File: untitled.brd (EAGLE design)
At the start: 100 x 100 mm, 16 parts, among them X2 pzem-004t

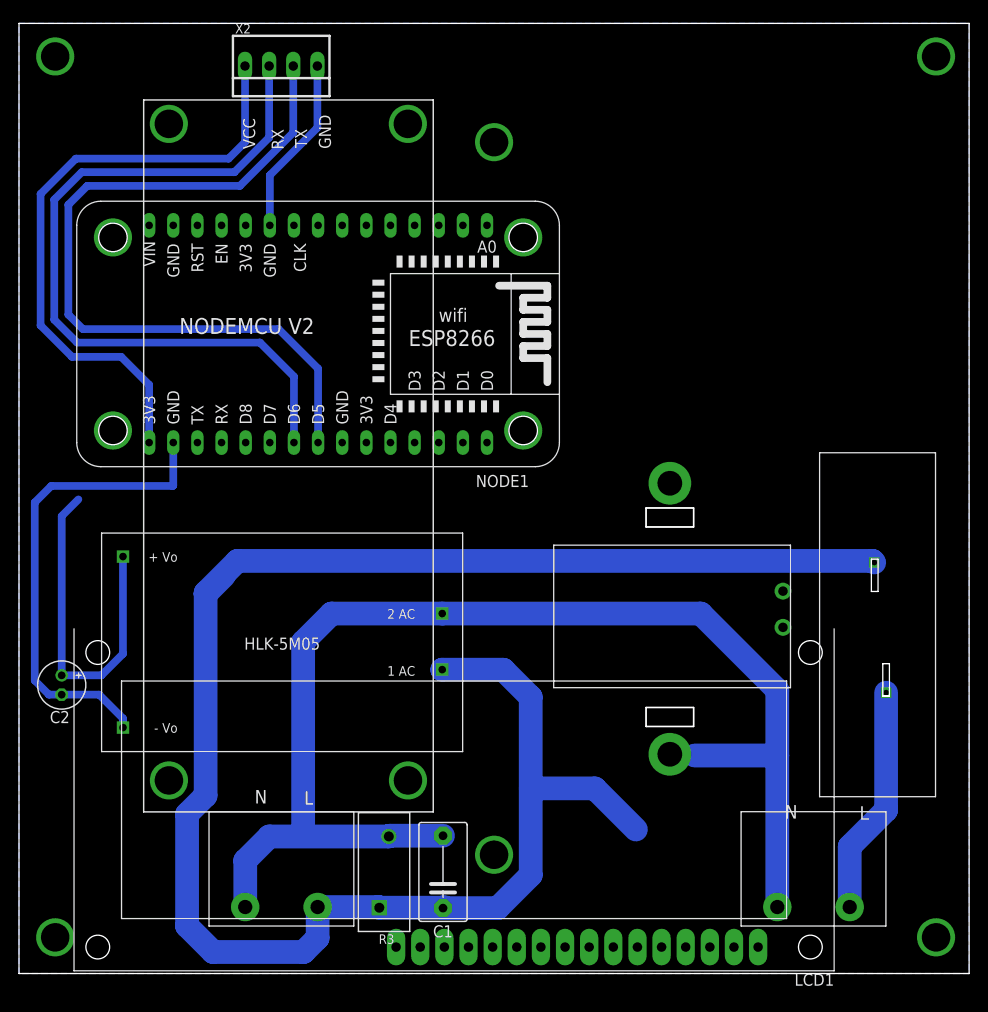
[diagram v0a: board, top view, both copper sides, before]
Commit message: 0021
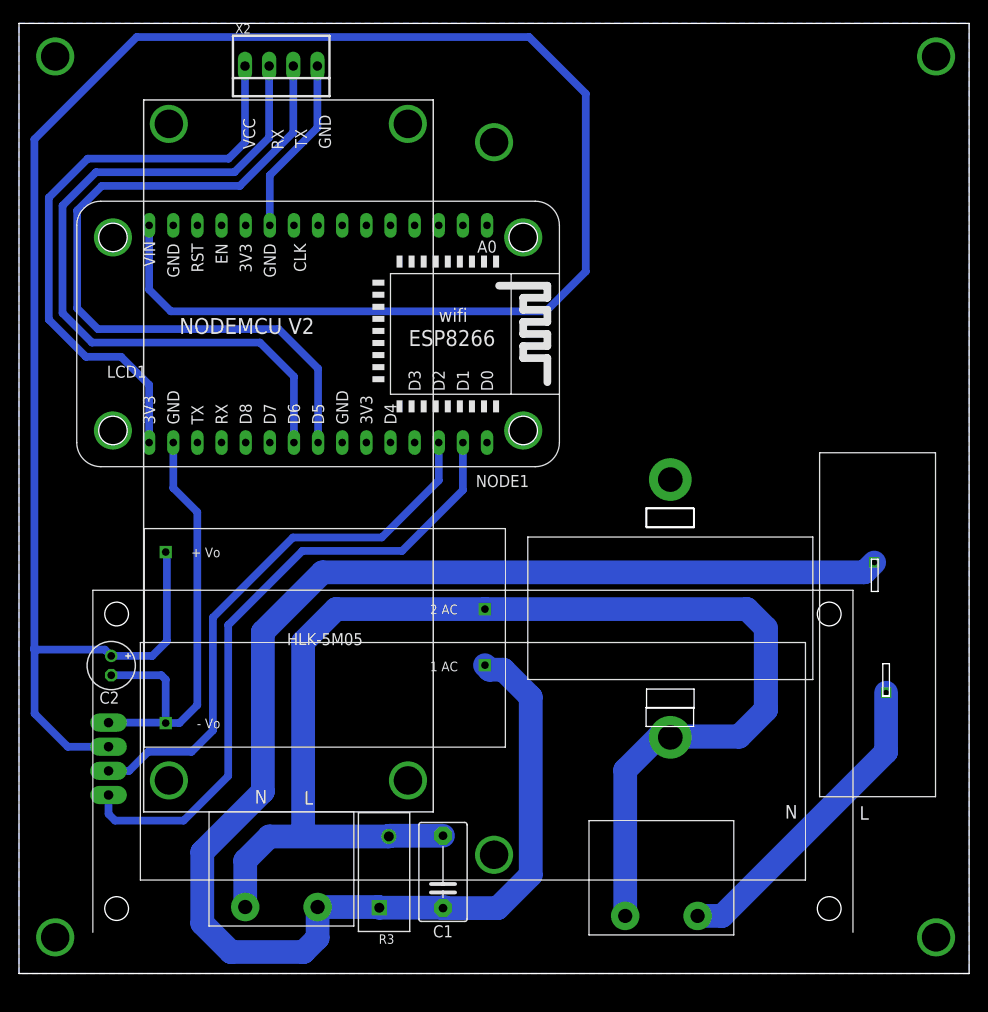
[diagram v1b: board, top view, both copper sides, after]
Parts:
- moved LCD1 75.7 mm to (13.2, 37.8), turned to 0 degrees
- moved 220 16.0 mm to (60.0, 4.06)
- moved C2 5.60 mm to (9.71, 32.4)
- moved U$1 4.52 mm to (32.2, 35.4)
- moved U$2 2.86 mm to (53.5, 30.9)
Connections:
- removed net VSS: LCD1.1
- new net SCL: LCD1.4, NODE1.D1
- new net SDA: LCD1.3, NODE1.D2
- net GND: now also LCD1.1
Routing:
- net VCC: track 36.9 -> 233.2 mm
- net SCL: track 0.00 -> 68.3 mm
- net SDA: track 0.00 -> 58.4 mm
- net N$7: track 195.4 -> 167.0 mm
- net N$9: track 24.1 -> 33.2 mm
- net N$21: track 132.7 -> 139.1 mm
- net TX: track 81.8 -> 79.2 mm
- net RX: track 80.1 -> 77.6 mm
- net 3V: track 65.7 -> 63.4 mm
- net GND: track 69.3 -> 68.2 mm
